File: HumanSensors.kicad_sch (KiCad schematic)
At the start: 0 parts

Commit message: Human sensors
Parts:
- added C1: 100n, lcsc_footprints:C5656610_MIC-SMD_6P-L3_5-W2_7-P0_90-BL, symbol Device:C
- added C2: 4,7u, symbol Device:C
- added C3: 100n, symbol Device:C
- added C4: 0,1u, lcsc_footprints:C5656610_MIC-SMD_6P-L3_5-W2_7-P0_90-BL, symbol Device:C
- added R1: 2K, lcsc_footprints:C37897213_SENSOR-TH_HLK-LD6002, symbol Device:R
- added R10: 100K, symbol Device:R
- added R6, R7, R9: 10K, symbol Device:R
- added R8: 10K, lcsc_footprints:C2848306_DFN-4_L1_5-W1_5-P0_8-TL-EP, symbol Device:R
- added U10: HLK-LD6002, lcsc_footprints:C37897213_SENSOR-TH_HLK-LD6002, symbol lcsc_imported:HLK-LD6002
- added U6: SCD40-D-R1, lcsc_footprints:C3037696_LGA-20_L10_1-W10_1-P1_25-TL, symbol lcsc_imported:SCD40-D-R1
- added U7: SHT40-AD1B-R3, lcsc_footprints:C2848306_DFN-4_L1_5-W1_5-P0_8-TL-EP, symbol lcsc_imported:SHT40-AD1B-R3
- added U8: ICS-43434_C5656610, lcsc_footprints:C5656610_MIC-SMD_6P-L3_5-W2_7-P0_90-BL, symbol lcsc_imported:ICS-43434_C5656610
- added U9: AM312, lcsc_footprints:C114881_TO-5-3_L8_2-W8_2, symbol lcsc_imported:AM312
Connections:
- new net: R1.2, U10.3 (P19)
- new net AC_BCLK: U8.4 (SCK)
- new net AC_RCLK: U8.1 (WS)
- new net CO2_SCL: R7.2, U6.9 (SCL)
- new net CO2_SDA: R6.2, U6.10 (SDA)
- new net D_IN: R10.1, U8.6 (SD)
- new net GND: C1.1, C2.1, C3.1, C4.2, R1.1, R10.2, U10.2 (GND), U6.21 (GND), U7.4 (VSS), U7.5 (EP), U8.2 (LR), U8.3 (GND), U9.3 (GND)
- new net PIR_OUT: U9.2 (OUT)
- new net R_RX0: U10.8 (RX0)
- new net R_TX0: U10.7 (TX0)
- new net Temp_SCL: R8.1, U7.2 (SCL)
- new net Temp_SDA: R9.1, U7.1 (SDA)
- new net VDD: C1.2, C2.2, C3.2, C4.1, R6.1, R7.1, R8.2, R9.2, U10.1 (3V3), U6.19 (VDDH), U6.7 (VDD), U7.3 (VDD), U8.5 (VDD), U9.1 (VCC)
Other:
- note added: "Acoustic Sensor"
- note added: "CO2 Sensor"
- note added: "PIR Sensor"
- note added: "Radar Sensor"
- note added: "Temp/humidity Sensor"

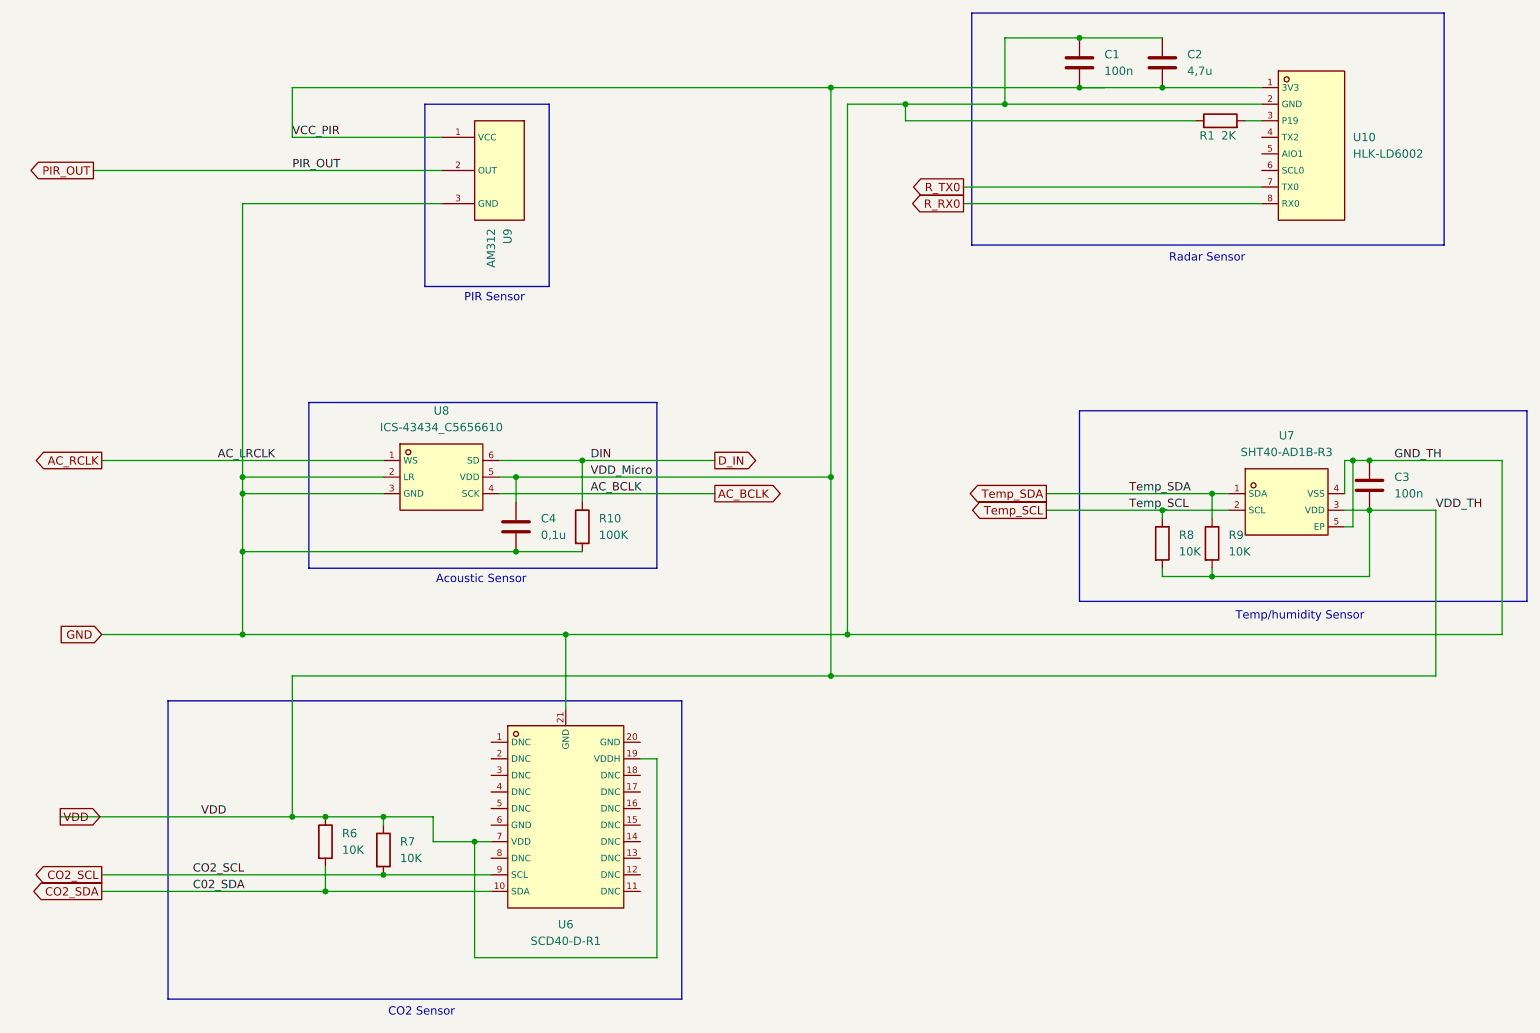
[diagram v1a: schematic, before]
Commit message: Rework MCU and Human sensor
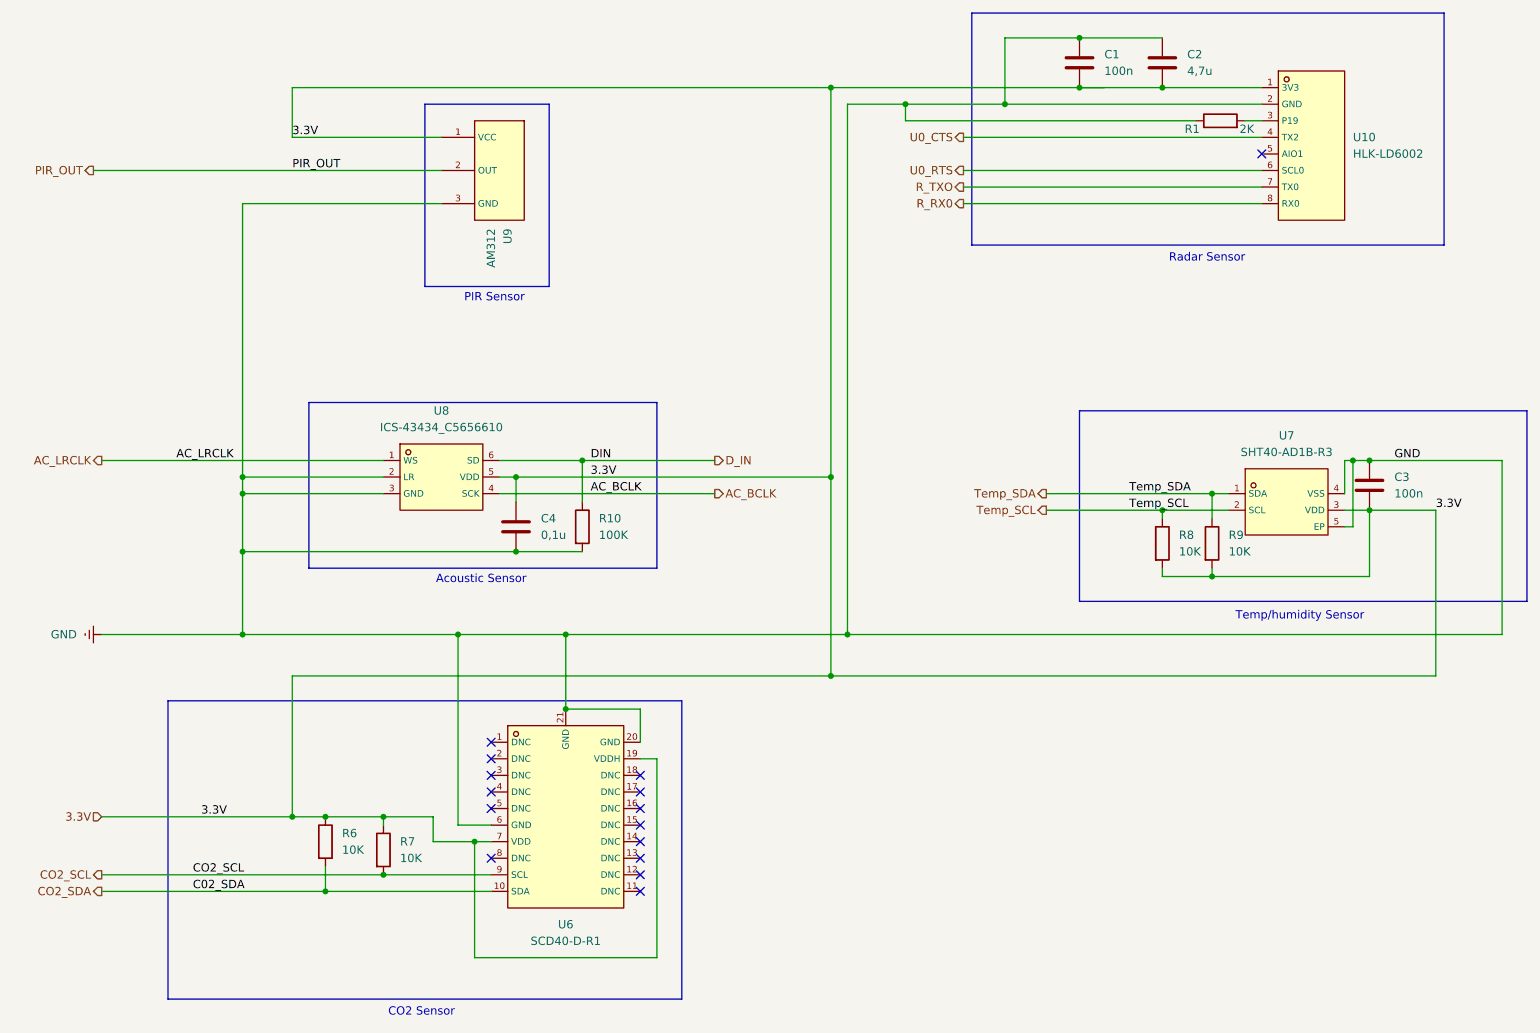
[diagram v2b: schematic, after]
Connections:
- net GND: now also U6.20 (GND), U6.6 (GND)
- net U0_CTS: now reaches U10.4 (TX2)
- net U0_RTS: now reaches U10.6 (SCL0)
- net AC_RCLK renamed AC_LRCLK
- net R_TX0 renamed R_TXO
- net VDD renamed 3.3V
- no-connect marks 0 -> 15
